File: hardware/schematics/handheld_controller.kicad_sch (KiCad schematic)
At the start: 0 parts

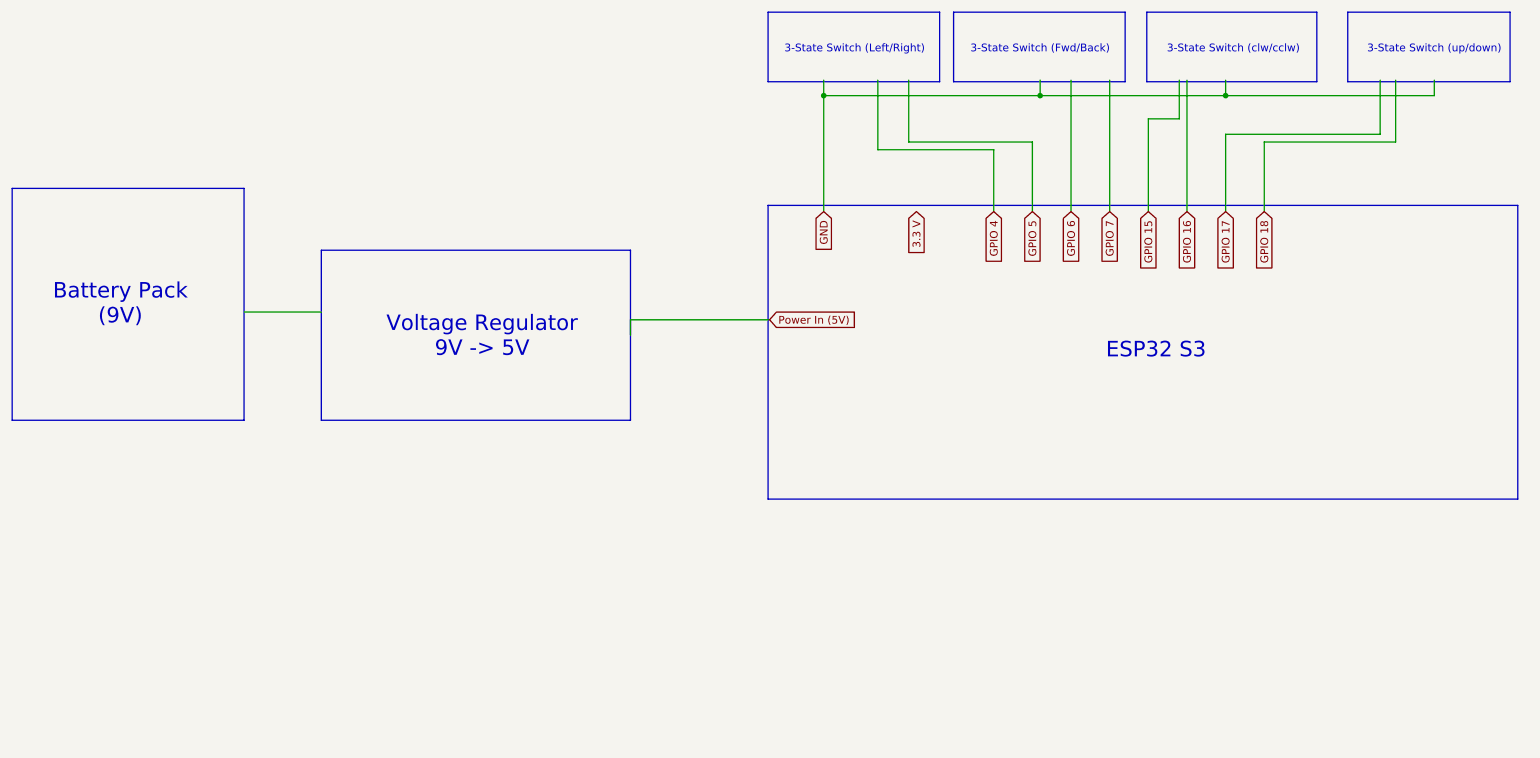
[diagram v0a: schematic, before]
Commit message: final (ish) schematic with real footprints
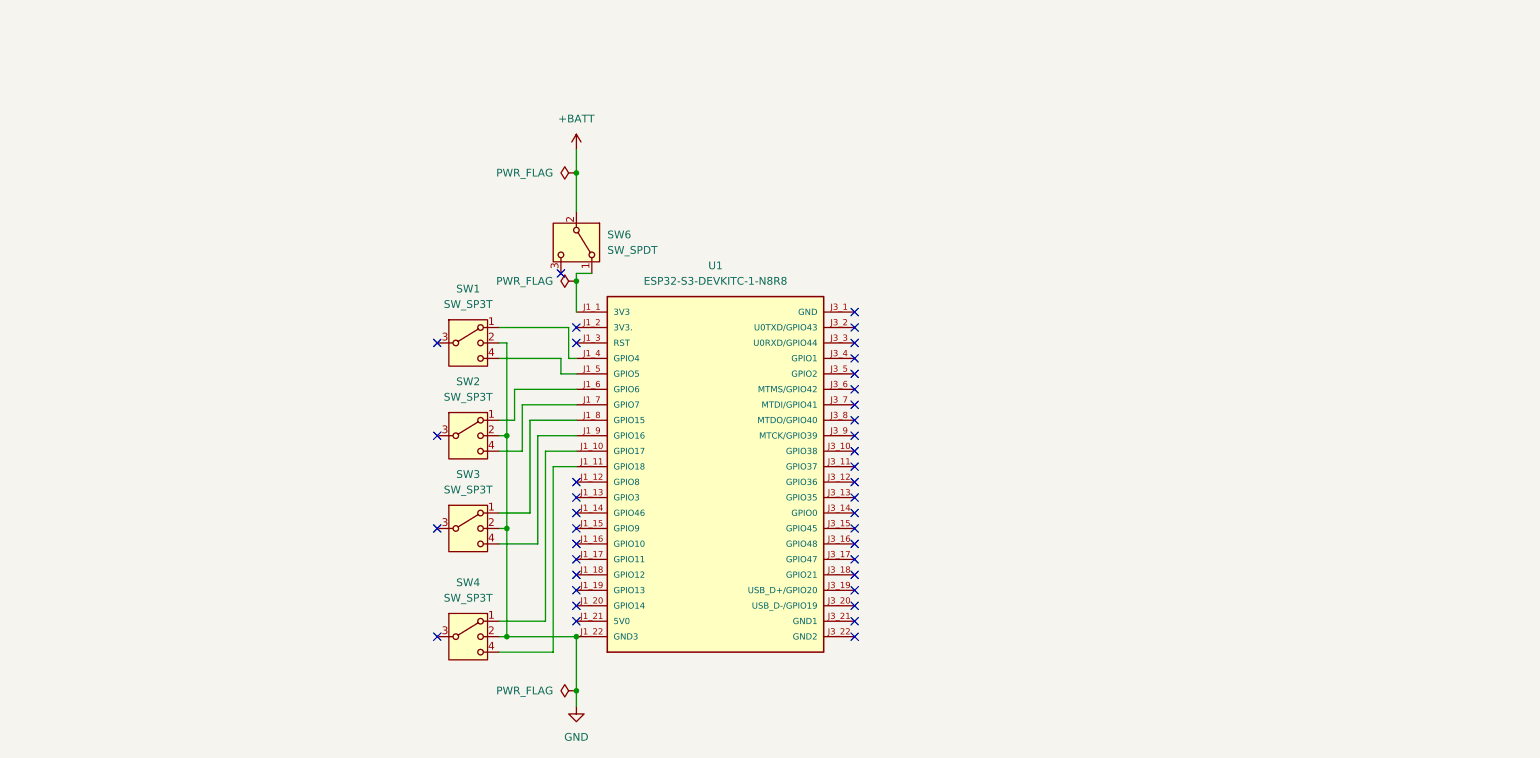
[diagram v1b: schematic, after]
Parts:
- added SW1, SW2, SW3, SW4: SW_SP3T, Button_Switch_SMD:SW_SP3T_PCM13, symbol Switch:SW_SP3T
- added SW6: SW_SPDT, Button_Switch_THT:SW_Lever_1P2T_NKK_GW12LxH, symbol Switch:SW_SPDT
- added U1: ESP32-S3-DEVKITC-1-N8R8, ESP32-S3-DEVKITC-1-N8R8:ESP32-S3-DEVKITC-1-N8R8, symbol ESP32-S3-DEVKITC-1-N8R8:ESP32-S3-DEVKITC-1-N8R8
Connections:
- net GND: now also SW1.2, SW2.2, SW3.2, SW4.2, U1.J1_22 (GND3)
- new net: SW1.1, U1.J1_4 (GPIO4)
- new net: SW1.4, U1.J1_5 (GPIO5)
- new net: SW2.1, U1.J1_6 (GPIO6)
- new net: SW2.4, U1.J1_7 (GPIO7)
- new net: SW6.1 (A), U1.J1_1 (3V3)
- new net: SW3.1, U1.J1_8 (GPIO15)
- new net: SW3.4, U1.J1_9 (GPIO16)
- new net: SW4.1, U1.J1_10 (GPIO17)
- new net: SW4.4, U1.J1_11 (GPIO18)
- new net +BATT: SW6.2 (B)
- no-connect marks 0 -> 39
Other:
- note removed: "3-State Switch (Fwd/Back)"
- note removed: "3-State Switch (Left/Right)"
- note removed: "3-State Switch (clw/cclw)"
- note removed: "3-State Switch (up/down)"
- note removed: "Battery Pack (9V)"
- note removed: "ESP32 S3"
- note removed: "Voltage Regulator 9V -> 5V"

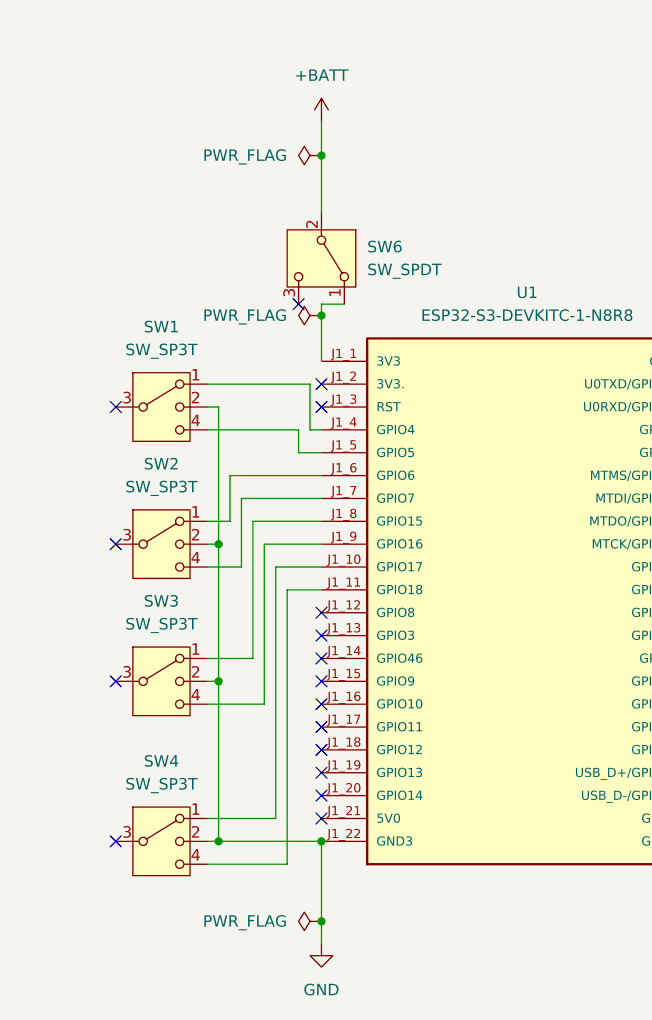
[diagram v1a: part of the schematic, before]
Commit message: acceptably final schematic (passes ERC)
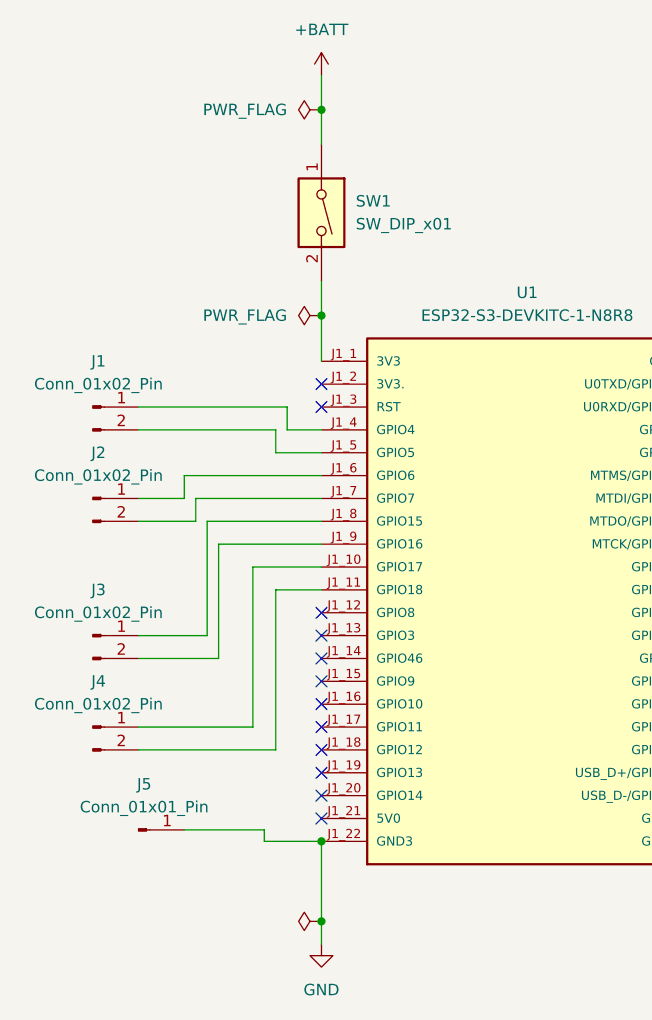
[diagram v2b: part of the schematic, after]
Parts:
- removed SW1, SW2, SW3, SW4: SW_SP3T, Button_Switch_SMD:SW_SP3T_PCM13, symbol Switch:SW_SP3T
- removed SW6: SW_SPDT, Button_Switch_THT:SW_Lever_1P2T_NKK_GW12LxH, symbol Switch:SW_SPDT
- added J1, J2, J3, J4: Conn_01x02_Pin, Connector_PinSocket_2.54mm:PinSocket_1x02_P2.54mm_Vertical, symbol Connector:Conn_01x02_Pin
- added J5: Conn_01x01_Pin, Connector_PinSocket_2.54mm:PinSocket_1x01_P2.54mm_Vertical, symbol Connector:Conn_01x01_Pin
- added SW1: SW_DIP_x01, Button_Switch_SMD:SW_SPST_SKQG_WithStem, symbol Switch:SW_DIP_x01
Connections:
- net +BATT: now also SW1.1
- net GND: now also J5.1 (Pin_1)
- net at U1.J1_4 (GPIO4): now also J1.1 (Pin_1)
- net at U1.J1_5 (GPIO5): now also J1.2 (Pin_2)
- net at U1.J1_6 (GPIO6): now also J2.1 (Pin_1)
- net at U1.J1_7 (GPIO7): now also J2.2 (Pin_2)
- net at U1.J1_1 (3V3): now also SW1.2
- net at U1.J1_8 (GPIO15): now also J3.1 (Pin_1)
- net at U1.J1_9 (GPIO16): now also J3.2 (Pin_2)
- net at U1.J1_10 (GPIO17): now also J4.1 (Pin_1)
- net at U1.J1_11 (GPIO18): now also J4.2 (Pin_2)
- no-connect marks 39 -> 34
